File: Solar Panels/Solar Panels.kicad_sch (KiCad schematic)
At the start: 58 parts, among them J2 5040500891

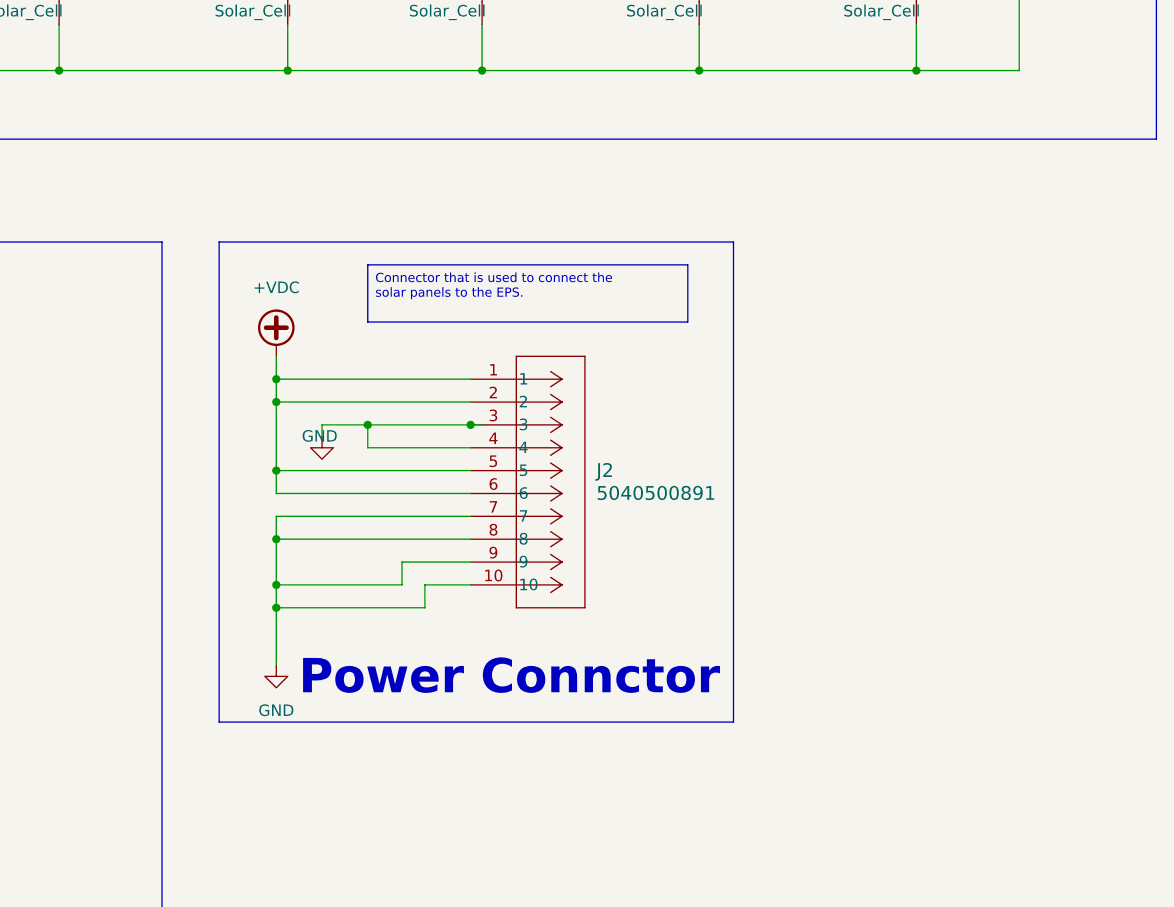
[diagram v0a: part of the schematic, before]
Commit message: Improve footprints, layout, routing
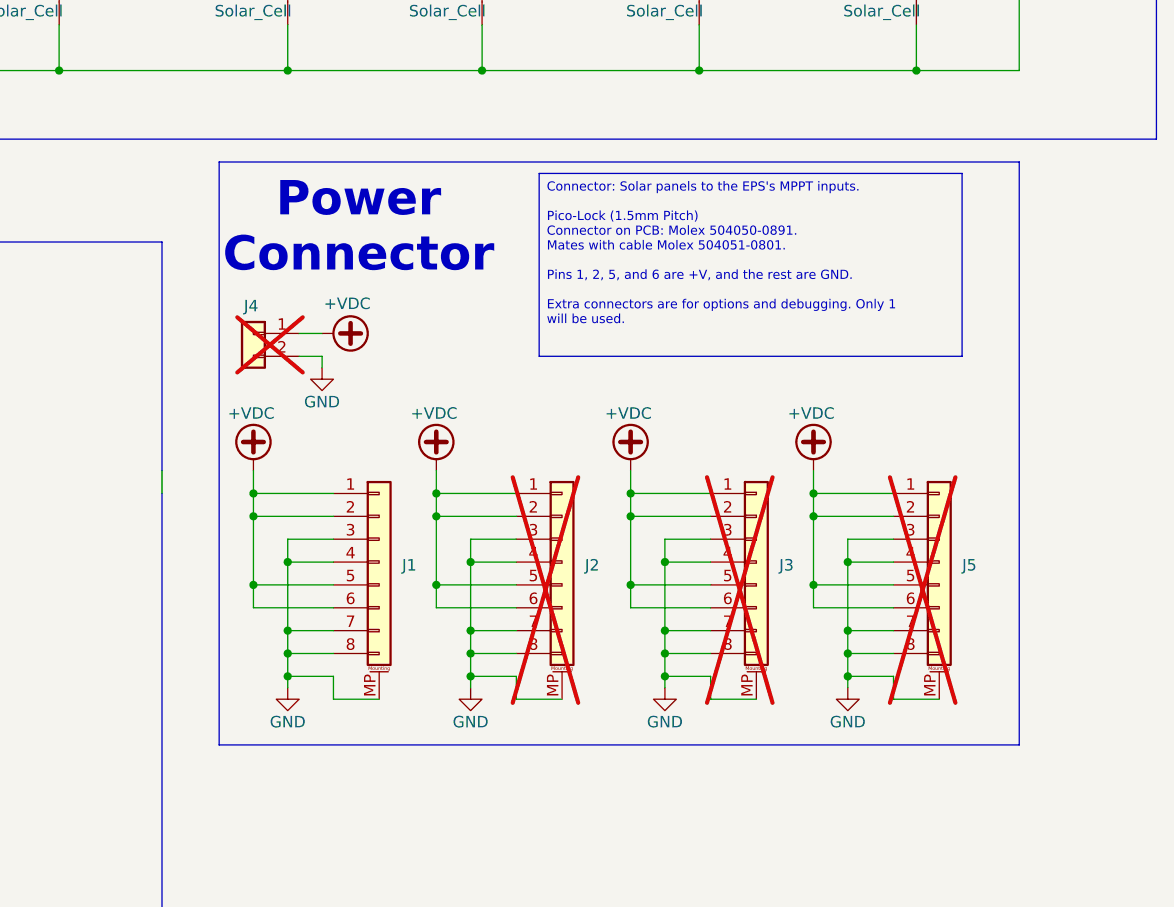
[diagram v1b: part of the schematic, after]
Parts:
- removed J2: 5040500891, Solar Panel Library:5040500891, symbol Calgary2Space:5040500891
- added J1, J2, J3: Conn_01x08_MountingPin, Connector_Molex:Molex_PicoBlade_53261-0871_1x08-1MP_P1.25mm_Horizontal, symbol Connector_Generic_MountingPin:Conn_01x08_MountingPin
- added J4: Conn_01x02, Connector_PinHeader_2.54mm:PinHeader_2x01_P2.54mm_Vertical, symbol Connector_Generic:Conn_01x02
- added J5: Conn_01x08_MountingPin, Connector_Molex:Molex_Pico-Lock_504050-0891_1x08-1MP_P1.50mm_Horizontal, symbol Connector_Generic_MountingPin:Conn_01x08_MountingPin
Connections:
- net +VDC: now also J1.1 (Pin_1), J1.2 (Pin_2), J1.5 (Pin_5), J1.6 (Pin_6), J2.1 (Pin_1), J2.2 (Pin_2), J2.5 (Pin_5), J2.6 (Pin_6), J3.1 (Pin_1), J3.2 (Pin_2), J3.5 (Pin_5), J3.6 (Pin_6), J4.1 (Pin_1), J5.1 (Pin_1), J5.2 (Pin_2), J5.5 (Pin_5), J5.6 (Pin_6)
- net GND: now also J1.3 (Pin_3), J1.4 (Pin_4), J1.7 (Pin_7), J1.8 (Pin_8), J1.MP (MountPin), J2.3 (Pin_3), J2.4 (Pin_4), J2.7 (Pin_7), J2.8 (Pin_8), J2.MP (MountPin), J3.3 (Pin_3), J3.4 (Pin_4), J3.7 (Pin_7), J3.8 (Pin_8), J3.MP (MountPin), J4.2 (Pin_2), J5.3 (Pin_3), J5.4 (Pin_4), J5.7 (Pin_7), J5.8 (Pin_8), J5.MP (MountPin)
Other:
- note added: "Power Connector"
- note removed: "Power Connctor"
- company: Calgary to Space -> CalgaryToSpace
- title: TriSolX Panels -> TriSolX 1.25U Solar Panel
